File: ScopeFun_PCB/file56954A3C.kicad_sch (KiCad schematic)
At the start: 10 parts, among them P1 USB3_TypeB, Q4 DMN6040SSD, U13 LTC4360-1

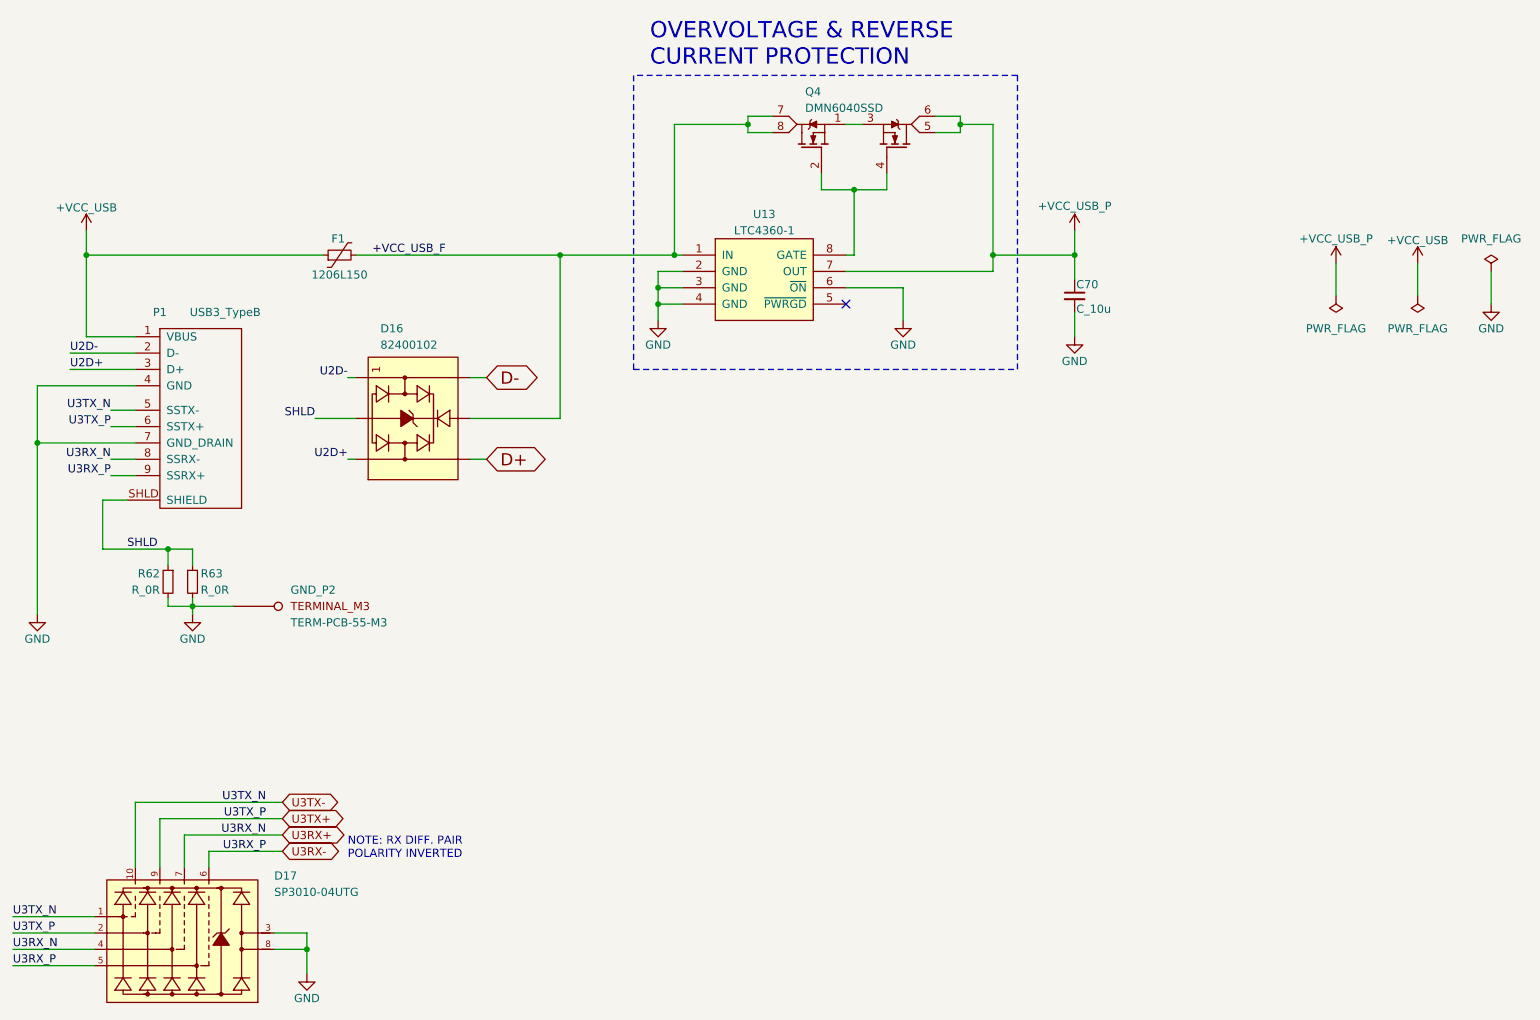
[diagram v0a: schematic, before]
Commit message: 0531
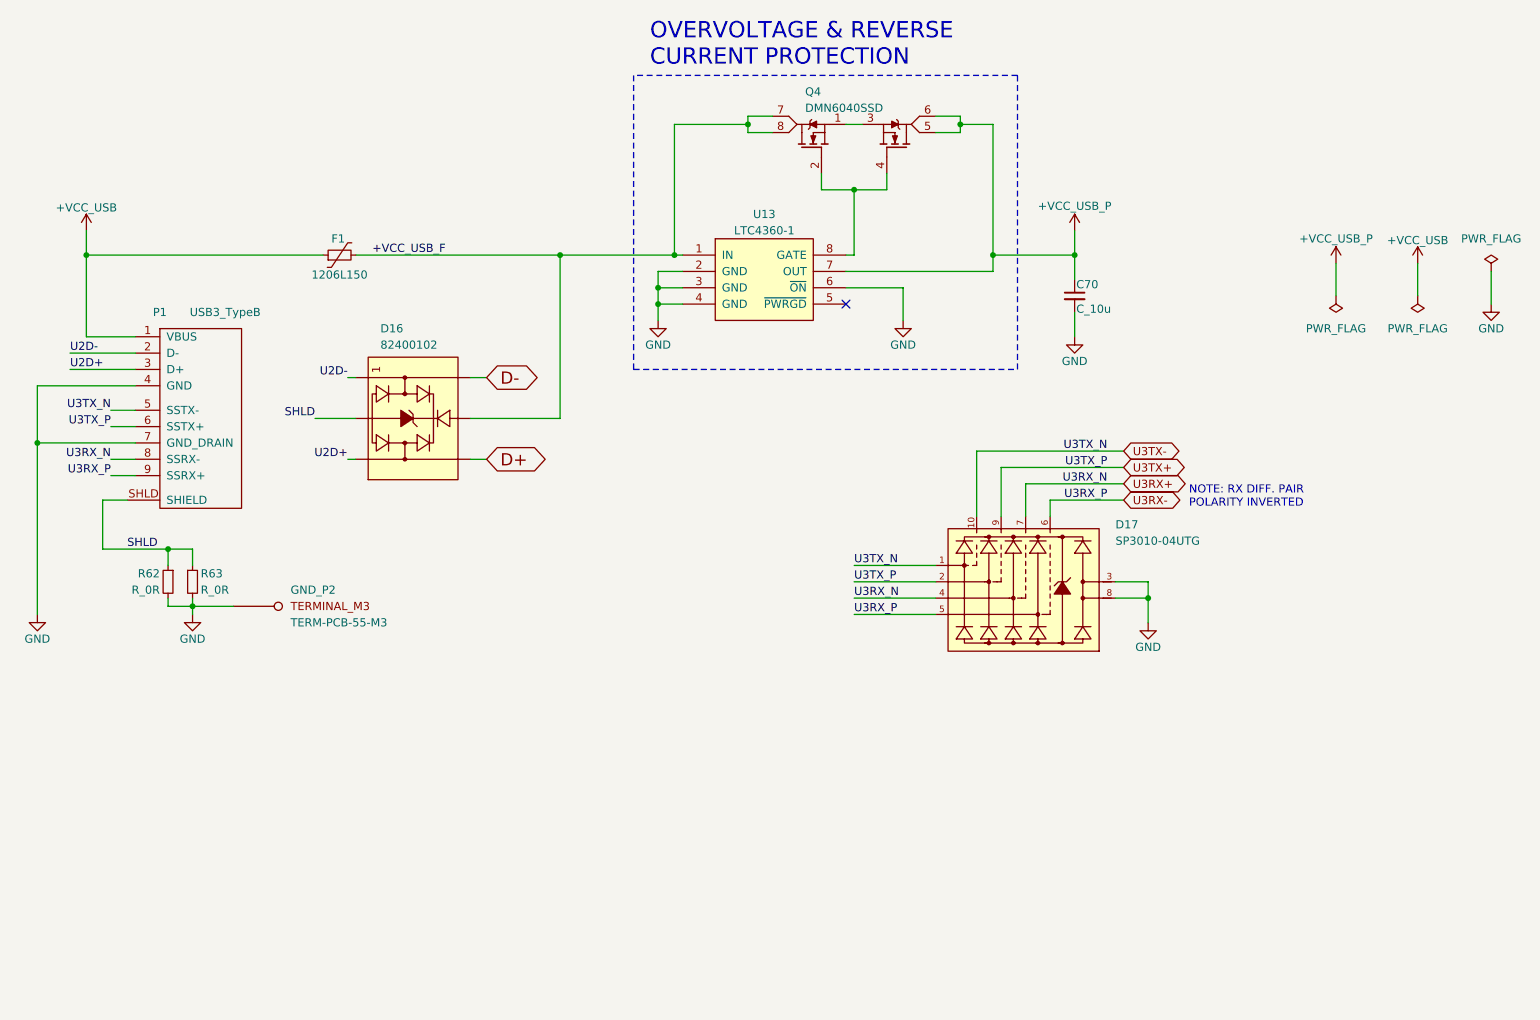
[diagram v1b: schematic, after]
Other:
- moved on the sheet: D17
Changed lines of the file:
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@@
 	(text "NOTE: RX DIFF. PAIR\nPOLARITY INVERTED"
 		(exclude_from_sim no)
-		(at 87.63 160.02 0)
+		(at 218.44 105.41 0)
 		(effects
 			(font
@@
 	)
 	(junction
-		(at 81.28 173.99)
+		(at 212.09 119.38)
 		(diameter 0)
 		(color 0 0 0 0)
@@
 	(wire
 		(pts
-			(xy 58.42 153.67) (xy 77.47 153.67)
+			(xy 189.23 99.06) (xy 208.28 99.06)
 		)
 		(stroke
@@
 	(wire
 		(pts
-			(xy 58.42 161.29) (xy 58.42 153.67)
+			(xy 189.23 106.68) (xy 189.23 99.06)
 		)
 		(stroke
@@
 	(wire
 		(pts
-			(xy 48.26 171.45) (xy 35.56 171.45)
+			(xy 179.07 116.84) (xy 166.37 116.84)
 		)
 		(stroke
@@
 	(wire
 		(pts
-			(xy 48.26 173.99) (xy 35.56 173.99)
+			(xy 179.07 119.38) (xy 166.37 119.38)
 		)
 		(stroke
@@
 	(wire
 		(pts
-			(xy 54.61 151.13) (xy 77.47 151.13)
+			(xy 185.42 96.52) (xy 208.28 96.52)
 		)
 		(stroke
@@
 	(wire
 		(pts
-			(xy 54.61 161.29) (xy 54.61 151.13)
+			(xy 185.42 106.68) (xy 185.42 96.52)
 		)
 		(stroke
@@
 	(wire
 		(pts
-			(xy 81.28 173.99) (xy 81.28 177.8)
+			(xy 212.09 119.38) (xy 212.09 123.19)
 		)
 		(stroke
@@
 	(wire
 		(pts
-			(xy 48.26 168.91) (xy 35.56 168.91)
+			(xy 179.07 114.3) (xy 166.37 114.3)
 		)
 		(stroke
@@
 	(wire
 		(pts
-			(xy 81.28 173.99) (xy 76.2 173.99)
+			(xy 212.09 119.38) (xy 207.01 119.38)
 		)
 		(stroke
@@
 	(wire
 		(pts
-			(xy 62.23 161.29) (xy 62.23 156.21)
-		)
-		(stroke
-			(width 0)
-			(type default)
-		)
-	)
-	(wire
-		(pts
-			(xy 81.28 171.45) (xy 81.28 173.99)
+			(xy 193.04 106.68) (xy 193.04 101.6)
+		)
+		(stroke
+			(width 0)
+			(type default)
+		)
+	)
+	(wire
+		(pts
+			(xy 212.09 116.84) (xy 212.09 119.38)
 		)
 		(stroke
@@
 	(wire
 		(pts
-			(xy 62.23 156.21) (xy 77.47 156.21)
+			(xy 193.04 101.6) (xy 208.28 101.6)
 		)
 		(stroke
@@
 	(wire
 		(pts
-			(xy 81.28 171.45) (xy 76.2 171.45)
+			(xy 212.09 116.84) (xy 207.01 116.84)
 		)
 		(stroke
@@
 	(wire
 		(pts
-			(xy 48.26 176.53) (xy 35.56 176.53)
-		)
-		(stroke
-			(width 0)
-			(type default)
-		)
-	)
-	(wire
-		(pts
-			(xy 66.04 158.75) (xy 77.47 158.75)
-		)
-		(stroke
-			(width 0)
-			(type default)
-		)
-	)
-	(wire
-		(pts
-			(xy 66.04 161.29) (xy 66.04 158.75)
+			(xy 179.07 121.92) (xy 166.37 121.92)
+		)
+		(stroke
+			(width 0)
+			(type default)
+		)
+	)
+	(wire
+		(pts
+			(xy 196.85 104.14) (xy 208.28 104.14)
+		)
+		(stroke
+			(width 0)
+			(type default)
+		)
+	)
+	(wire
+		(pts
+			(xy 196.85 106.68) (xy 196.85 104.14)
 		)
 		(stroke
@@
 	)
 	(label "U3TX_P"
-		(at 35.56 171.45 0)
+		(at 166.37 116.84 0)
 		(effects
 			(font
@@
 	)
 	(label "U3RX_N"
-		(at 35.56 173.99 0)
+		(at 166.37 119.38 0)
 		(effects
 			(font
@@
 	)
 	(label "U3TX_N"
-		(at 35.56 168.91 0)
+		(at 166.37 114.3 0)
 		(effects
 			(font
@@
 	)
 	(label "U3RX_P"
-		(at 74.93 158.75 180)
+		(at 205.74 104.14 180)
 		(effects
 			(font
@@
 	)
 	(label "U3TX_P"
-		(at 74.93 153.67 180)
+		(at 205.74 99.06 180)
 		(effects
 			(font
@@
 	)
 	(label "U3RX_P"
-		(at 35.56 176.53 0)
+		(at 166.37 121.92 0)
 		(effects
 			(font
@@
 	)
 	(label "U3TX_N"
-		(at 74.93 151.13 180)
+		(at 205.74 96.52 180)
 		(effects
 			(font
@@
 	)
 	(label "U3RX_N"
-		(at 74.93 156.21 180)
+		(at 205.74 101.6 180)
 		(effects
 			(font
@@
 	(global_label "U3RX-"
 		(shape bidirectional)
-		(at 77.47 158.75 0)
+		(at 208.28 104.14 0)
 		(effects
 			(font
@@
 		)
 		(property "Intersheetrefs" "${INTERSHEET_REFS}"
-			(at 77.47 158.75 0)
+			(at 208.28 104.14 0)
 			(hide yes)
 			(show_name no)
@@
 	(global_label "U3TX-"
 		(shape bidirectional)
-		(at 77.47 151.13 0)
+		(at 208.28 96.52 0)
 		(effects
 			(font
@@
 		)
 		(property "Intersheetrefs" "${INTERSHEET_REFS}"
-			(at 77.47 151.13 0)
+			(at 208.28 96.52 0)
 			(hide yes)
 			(show_name no)
@@
 	(global_label "U3TX+"
 		(shape bidirectional)
-		(at 77.47 153.67 0)
+		(at 208.28 99.06 0)
 		(effects
 			(font
@@
 		)
 		(property "Intersheetrefs" "${INTERSHEET_REFS}"
-			(at 77.47 153.67 0)
+			(at 208.28 99.06 0)
 			(hide yes)
 			(show_name no)
@@
 	(global_label "U3RX+"
 		(shape bidirectional)
-		(at 77.47 156.21 0)
+		(at 208.28 101.6 0)
 		(effects
 			(font
@@
 		)
 		(property "Intersheetrefs" "${INTERSHEET_REFS}"
-			(at 77.47 156.21 0)
+			(at 208.28 101.6 0)
 			(hide yes)
 			(show_name no)
@@
 	(symbol
 		(lib_id "ScopefunParts:SP3010-04UTG")
-		(at 62.23 172.72 0)
+		(at 193.04 118.11 0)
 		(unit 1)
 		(body_style 1)
@@
 		(dnp no)
 		(property "Reference" "D17"
-			(at 76.2 162.56 0)
+			(at 207.01 107.95 0)
 			(show_name no)
 			(do_not_autoplace no)
@@
 		)
 		(property "Value" "SP3010-04UTG"
-			(at 76.2 165.1 0)
+			(at 207.01 110.49 0)
 			(show_name no)
 			(do_not_autoplace no)
@@
 		)
 		(property "Footprint" "ScopefunPackagesLibrary:uDFN-10"
-			(at 61.214 184.658 0)
+			(at 192.024 130.048 0)
 			(hide yes)
 			(show_name no)
@@
 		)
 		(property "Datasheet" "http://www.littelfuse.com/~/media/electronics/datasheets/tvs_diode_arrays/littelfuse_tvs_diode_array_sp3010_datasheet.pdf.pdf"
-			(at 61.214 187.198 0)
+			(at 192.024 132.588 0)
 			(hide yes)
 			(show_name no)
@@
 		)
 		(property "Description" "SP3010 Series 0.45pF Diode Array"
-			(at 62.23 156.21 0)
+			(at 193.04 101.6 0)
 			(hide yes)
 			(show_name no)
@@
 		)
 		(property "MFG Part#" "SP3010-04UTG"
-			(at 62.23 158.75 0)
+			(at 193.04 104.14 0)
 			(hide yes)
 			(show_name no)
@@
 		(lib_name "GND_9")
 		(lib_id "Scopefun_v2-rescue:GND")
-		(at 81.28 177.8 0)
+		(at 212.09 123.19 0)
 		(unit 1)
 		(body_style 1)
@@
 		(dnp no)
 		(property "Reference" "#PWR0124"
-			(at 81.28 184.15 0)
+			(at 212.09 129.54 0)
 			(hide yes)
 			(show_name no)
@@
 		)
 		(property "Value" "GND"
-			(at 81.28 181.61 0)
+			(at 212.09 127 0)
 			(show_name no)
 			(do_not_autoplace no)
@@
 		)
 		(property "Footprint" ""
-			(at 81.28 177.8 0)
+			(at 212.09 123.19 0)
 			(show_name no)
 			(do_not_autoplace no)
@@
 		)
 		(property "Datasheet" ""
-			(at 81.28 177.8 0)
+			(at 212.09 123.19 0)
 			(show_name no)
 			(do_not_autoplace no)
@@
 		)
 		(property "Description" ""
-			(at 81.28 177.8 0)
-			(show_name no)
-			(do_not_autoplace no)
+			(at 212.09 123.19 0)
+			(show_name no)
+			(do_not_autoplace no)
